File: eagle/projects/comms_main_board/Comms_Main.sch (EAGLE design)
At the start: 53 parts, among them J1 RECE-20279-001E, Q1 CSD17579Q3A, U1 TPS562209DDCT, U2 LP2985-33DBVR, U3 LP5900TLX-3.3/NOPB, U4 TPS562209DDCT, U5 LMZ34002RKGR, U6 LM3488MMX/NOPB

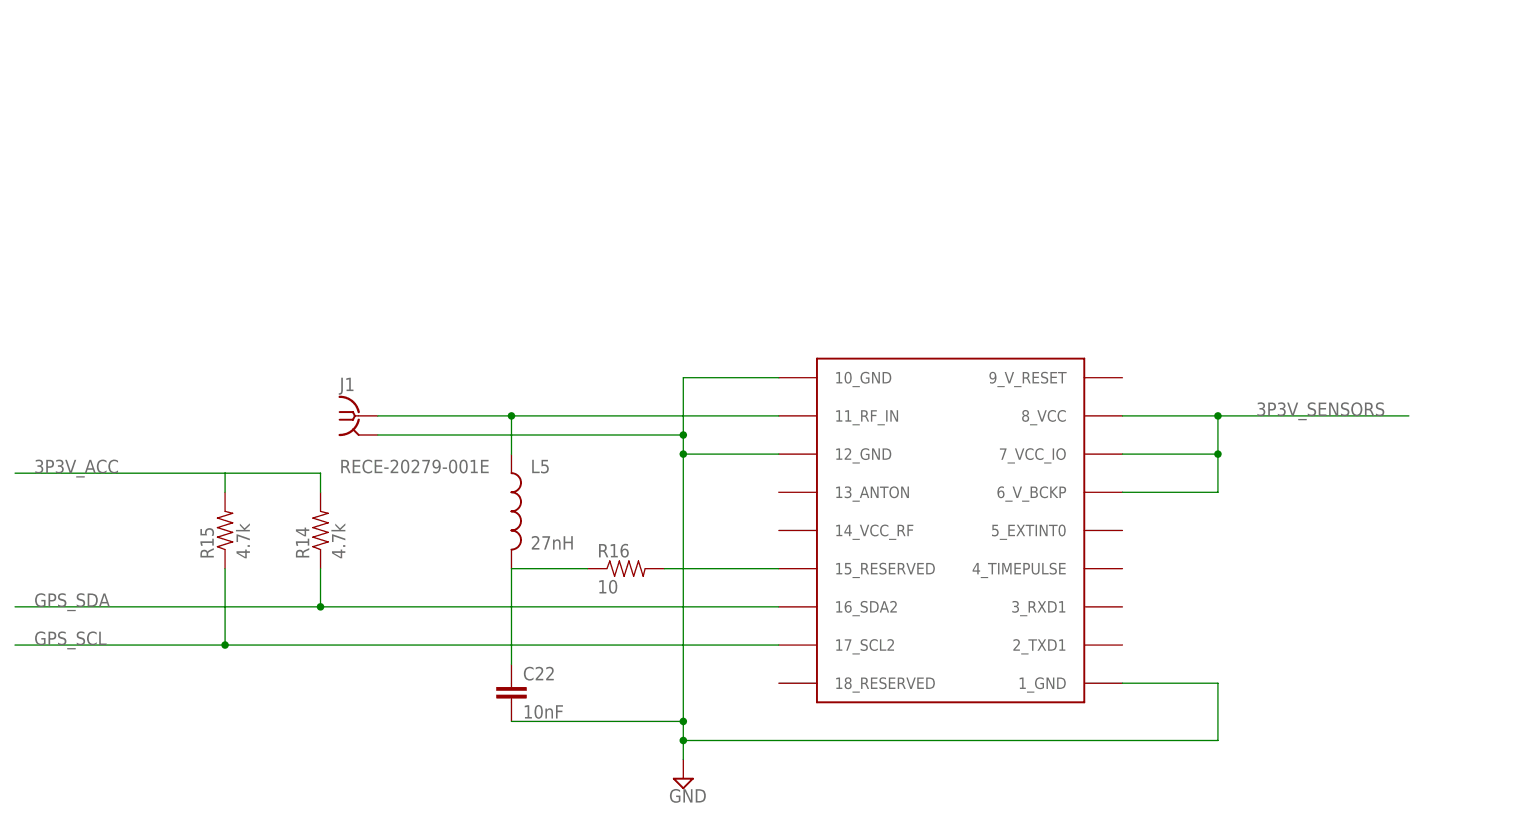
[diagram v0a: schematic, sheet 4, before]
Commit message: Finishing touches to GPS schematic
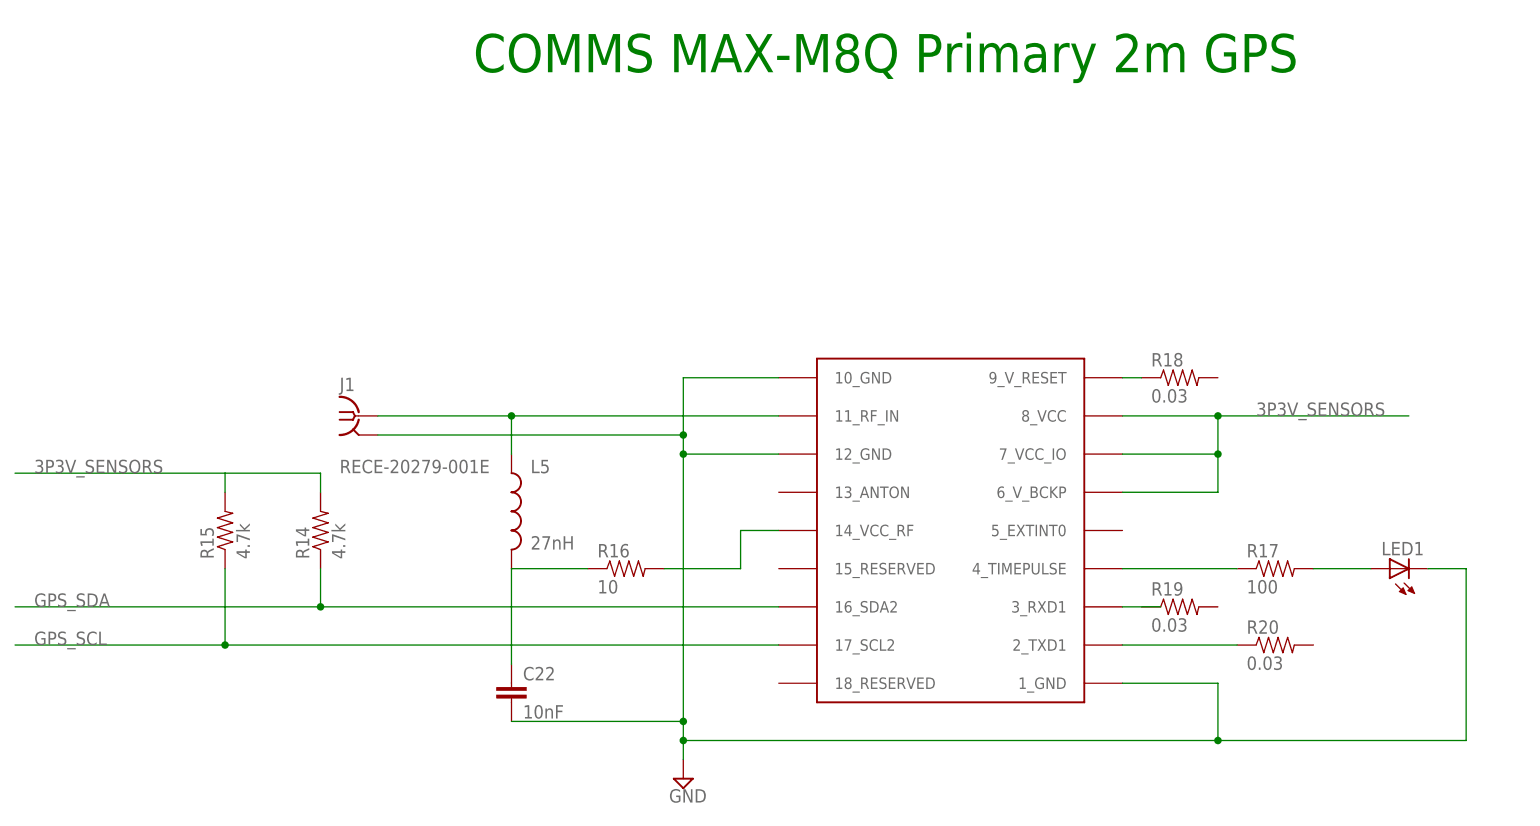
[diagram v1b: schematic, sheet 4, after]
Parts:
- added LED1: (no value), comms:LEDCHIP-LED0805
- added R17: 100, comms:RES_0R100_0603
- added R18, R19, R20: 0.03, comms:RES_0RS030_0805
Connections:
- removed net 3P3V_ACC: R14.2, R15.2
- new net N$23: R17.1, U$1.4_TIMEPULSE
- new net N$25: LED1.A, R17.2
- new net N$26: U$1.3_RXD1
- new net N$27: R20.1, U$1.2_TXD1
- new net N$28: R18.1, U$1.9_V_RESET
- net 3P3V_SENSORS: now also R14.2, R15.2
- net GND: now also LED1.C
- net N$20: now also U$1.14_VCC_RF; no longer U$1.15_RESERVED
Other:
- note added: "COMMS MAX-M8Q Primary 2m GPS"
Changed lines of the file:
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@@
 <part name="C22" library="comms" deviceset="CAP" device="_0805" technology="_10NF0" value="10nF"/>
 <part name="L5" library="comms" deviceset="L" device="_0603" technology="_27NH0" value="27nH"/>
+<part name="R17" library="comms" deviceset="RES" device="_0603" technology="_0R100" value="100"/>
+<part name="LED1" library="comms" deviceset="LED" device="CHIP-LED0805"/>
+<part name="R19" library="comms" deviceset="RES" device="_0805" technology="_0RS030" value="0.03"/>
+<part name="R20" library="comms" deviceset="RES" device="_0805" technology="_0RS030" value="0.03"/>
+<part name="R18" library="comms" deviceset="RES" device="_0805" technology="_0RS030" value="0.03"/>
 </parts>
 <sheets>
@@
 <sheet>
 <plain>
+<text x="71.12" y="162.56" size="5.08" layer="91">COMMS MAX-M8Q Primary 2m GPS</text>
 </plain>
 <instances>
@@
 <instance part="C22" gate="G$1" x="76.2" y="78.74"/>
 <instance part="L5" gate="G$1" x="76.2" y="104.14"/>
+<instance part="R17" gate="G$1" x="177.8" y="96.52"/>
+<instance part="LED1" gate="G$1" x="193.04" y="96.52" rot="R90"/>
+<instance part="R19" gate="G$1" x="165.1" y="91.44"/>
+<instance part="R20" gate="G$1" x="177.8" y="86.36"/>
+<instance part="R18" gate="G$1" x="165.1" y="121.92"/>
 </instances>
 <busses>
@@
 <junction x="170.18" y="111.76"/>
 </segment>
-</net>
-<net name="3P3V_ACC" class="0">
 <segment>
 <pinref part="R15" gate="G$1" pin="2"/>
@@
 <wire x1="76.2" y1="76.2" x2="99.06" y2="76.2" width="0.1524" layer="91"/>
 <junction x="99.06" y="76.2"/>
+<pinref part="LED1" gate="G$1" pin="C"/>
+<wire x1="198.12" y1="96.52" x2="203.2" y2="96.52" width="0.1524" layer="91"/>
+<wire x1="203.2" y1="96.52" x2="203.2" y2="73.66" width="0.1524" layer="91"/>
+<wire x1="203.2" y1="73.66" x2="170.18" y2="73.66" width="0.1524" layer="91"/>
+<junction x="170.18" y="73.66"/>
 </segment>
 </net>
@@
 </segment>
 </net>
+<net name="N$23" class="0">
+<segment>
+<pinref part="U$1" gate="G$1" pin="4_TIMEPULSE"/>
+<pinref part="R17" gate="G$1" pin="1"/>
+<wire x1="157.48" y1="96.52" x2="172.72" y2="96.52" width="0.1524" layer="91"/>
+</segment>
+</net>
+<net name="N$25" class="0">
+<segment>
+<pinref part="R17" gate="G$1" pin="2"/>
+<pinref part="LED1" gate="G$1" pin="A"/>
+<wire x1="182.88" y1="96.52" x2="190.5" y2="96.52" width="0.1524" layer="91"/>
+</segment>
+</net>
+<net name="N$26" class="0">
+<segment>
+<pinref part="U$1" gate="G$1" pin="3_RXD1"/>
+<wire x1="157.48" y1="91.44" x2="162.56" y2="91.44" width="0.1524" layer="91"/>
+</segment>
+</net>
+<net name="N$27" class="0">
+<segment>
+<pinref part="U$1" gate="G$1" pin="2_TXD1"/>
+<pinref part="R20" gate="G$1" pin="1"/>
+<wire x1="157.48" y1="86.36" x2="172.72" y2="86.36" width="0.1524" layer="91"/>
+</segment>
+</net>
+<net name="N$28" class="0">
+<segment>
+<pinref part="U$1" gate="G$1" pin="9_V_RESET"/>
+<pinref part="R18" gate="G$1" pin="1"/>
+<wire x1="157.48" y1="121.92" x2="160.02" y2="121.92" width="0.1524" layer="91"/>
+</segment>
+</net>
 <net name="N$20" class="0">
 <segment>
+<pinref part="U$1" gate="G$1" pin="14_VCC_RF"/>
+<wire x1="111.76" y1="101.6" x2="106.68" y2="101.6" width="0.1524" layer="91"/>
+<wire x1="106.68" y1="101.6" x2="106.68" y2="96.52" width="0.1524" layer="91"/>
 <pinref part="R16" gate="G$1" pin="2"/>
-<pinref part="U$1" gate="G$1" pin="15_RESERVED"/>
-<wire x1="96.52" y1="96.52" x2="111.76" y2="96.52" width="0.1524" layer="91"/>
-</segment>
-</net>
+<wire x1="106.68" y1="96.52" x2="96.52" y2="96.52" width="0.1524" layer="91"/>
+</segment>
+</net>
